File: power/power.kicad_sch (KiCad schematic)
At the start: 32 parts, among them J1 ET60T-D04-3-08-D04-X-R1-S, J2 796636-6, J3 misc. power output, J4 misc. power output, J5 misc. power output, J7 misc. power output

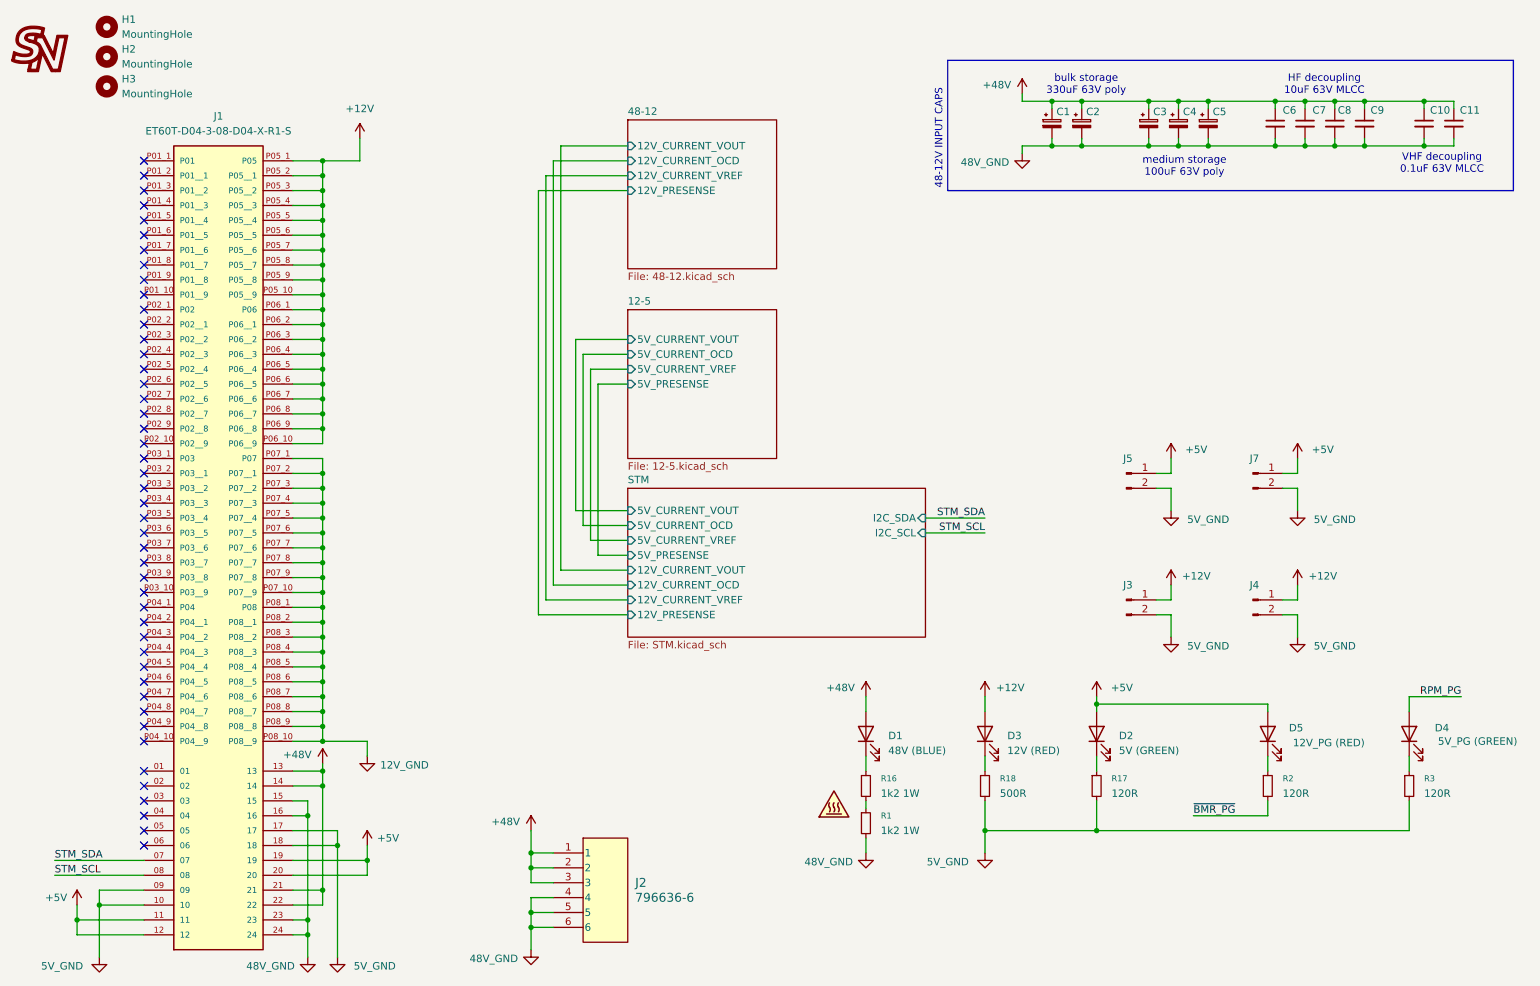
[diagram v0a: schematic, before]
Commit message: work
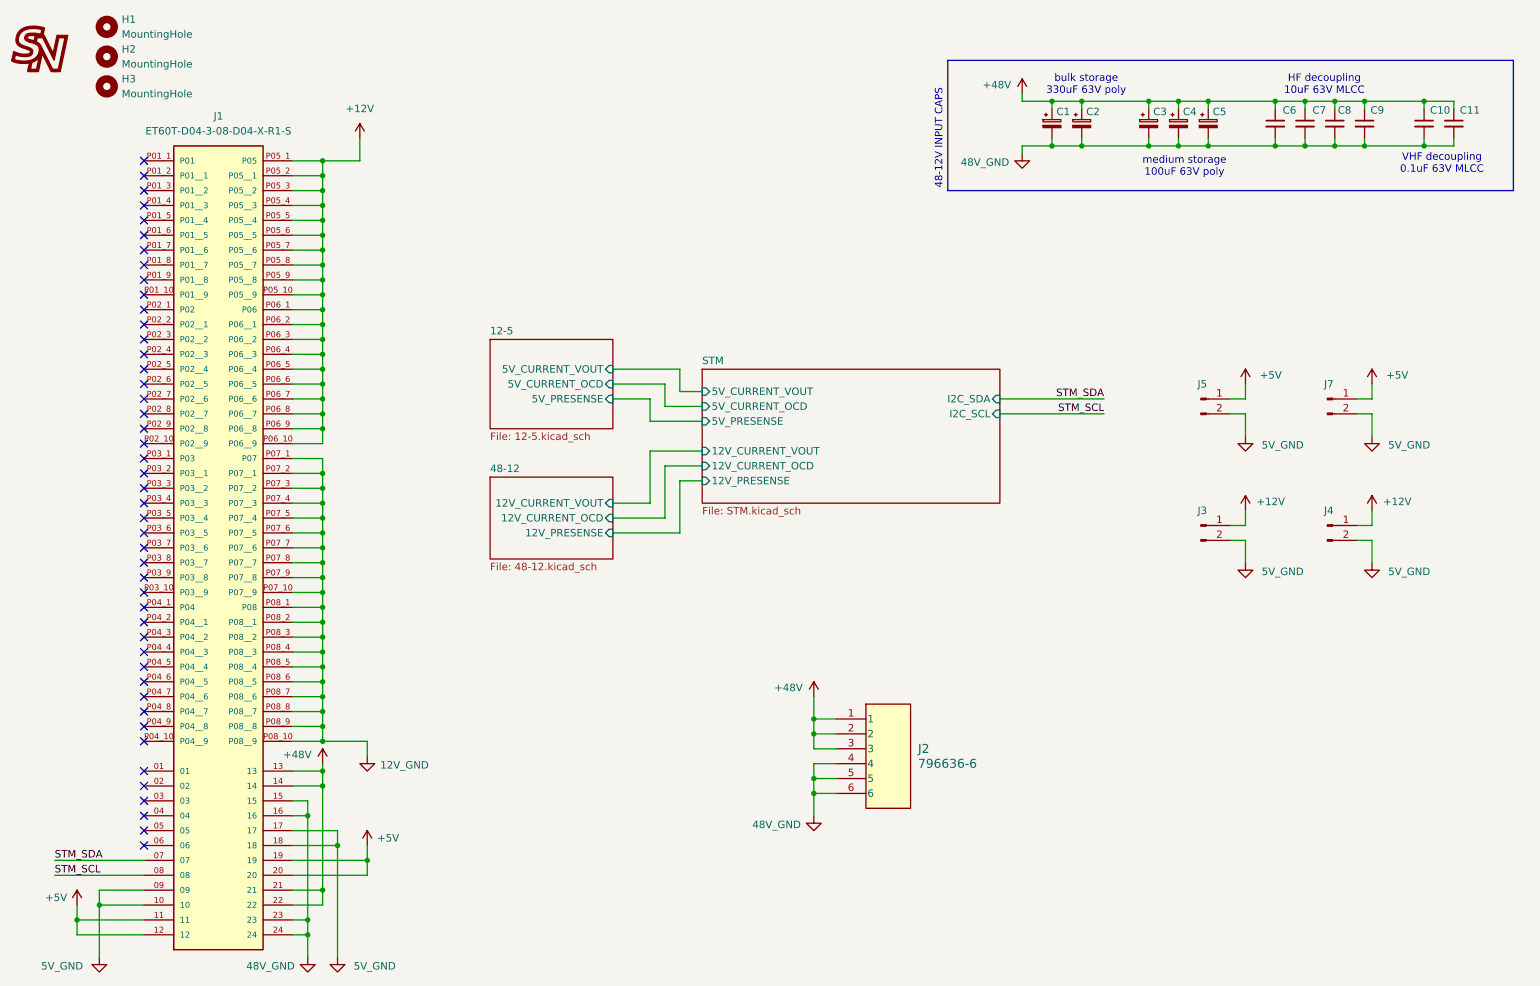
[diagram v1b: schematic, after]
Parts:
- removed D1: 48V (BLUE), symbol Device:LED
- removed D2: 5V (GREEN), symbol Device:LED
- removed D3: 12V (RED), symbol Device:LED
- removed D4: 5V_PG (GREEN), symbol Device:LED
- removed D5: 12V_PG (RED), symbol Device:LED
- removed R1, R16: 1k2 1W, symbol Device:R_Small
- removed R17, R2, R3: 120R, symbol Device:R_Small
- removed R18: 500R, symbol Device:R_Small
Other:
- sheet 12-5 ports: added none; removed 5V_CURRENT_VREF
- sheet 48-12 ports: added none; removed 12V_CURRENT_VREF
- sheet STM ports: added none; removed 12V_CURRENT_VREF, 5V_CURRENT_VREF
- moved on the sheet: J2, J3, J4, J5, J7
